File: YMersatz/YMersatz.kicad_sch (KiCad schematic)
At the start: 9 parts, among them J1 Conn_01x20, J2 Conn_01x20, U1 74LS574, U2 74LS08, Y1 SG-615

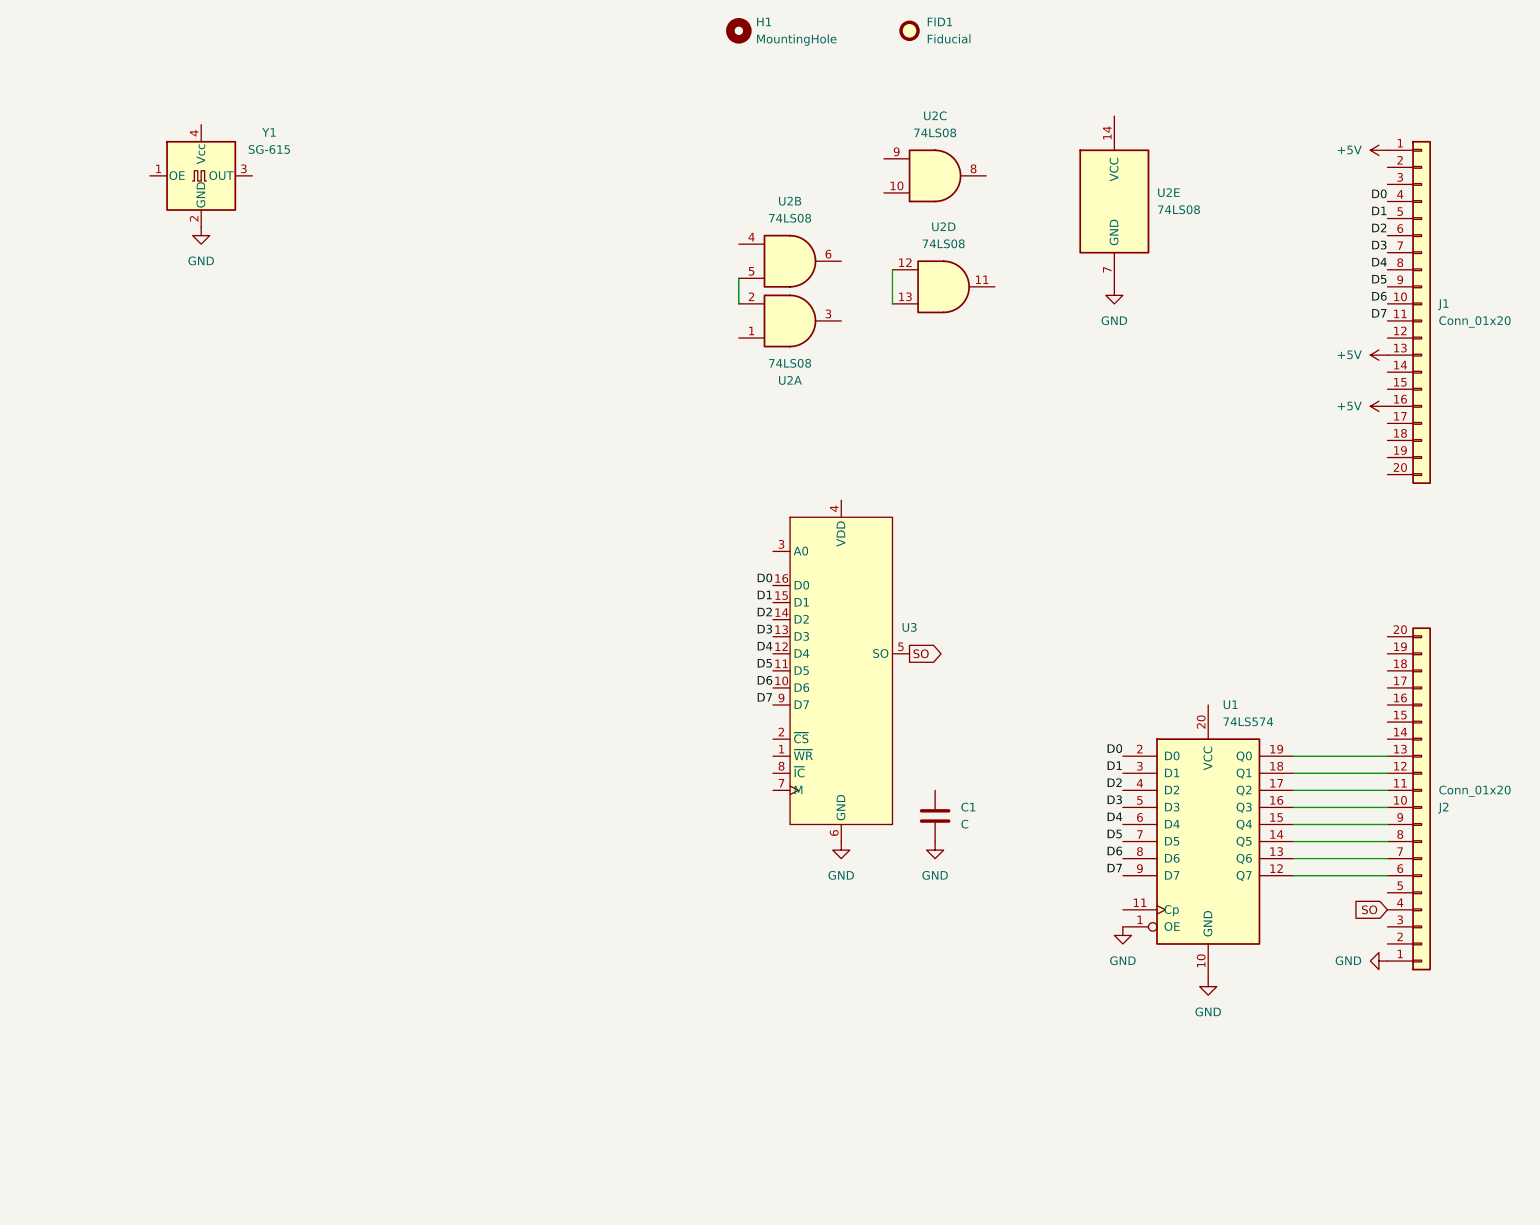
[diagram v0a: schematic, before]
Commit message: ym pins
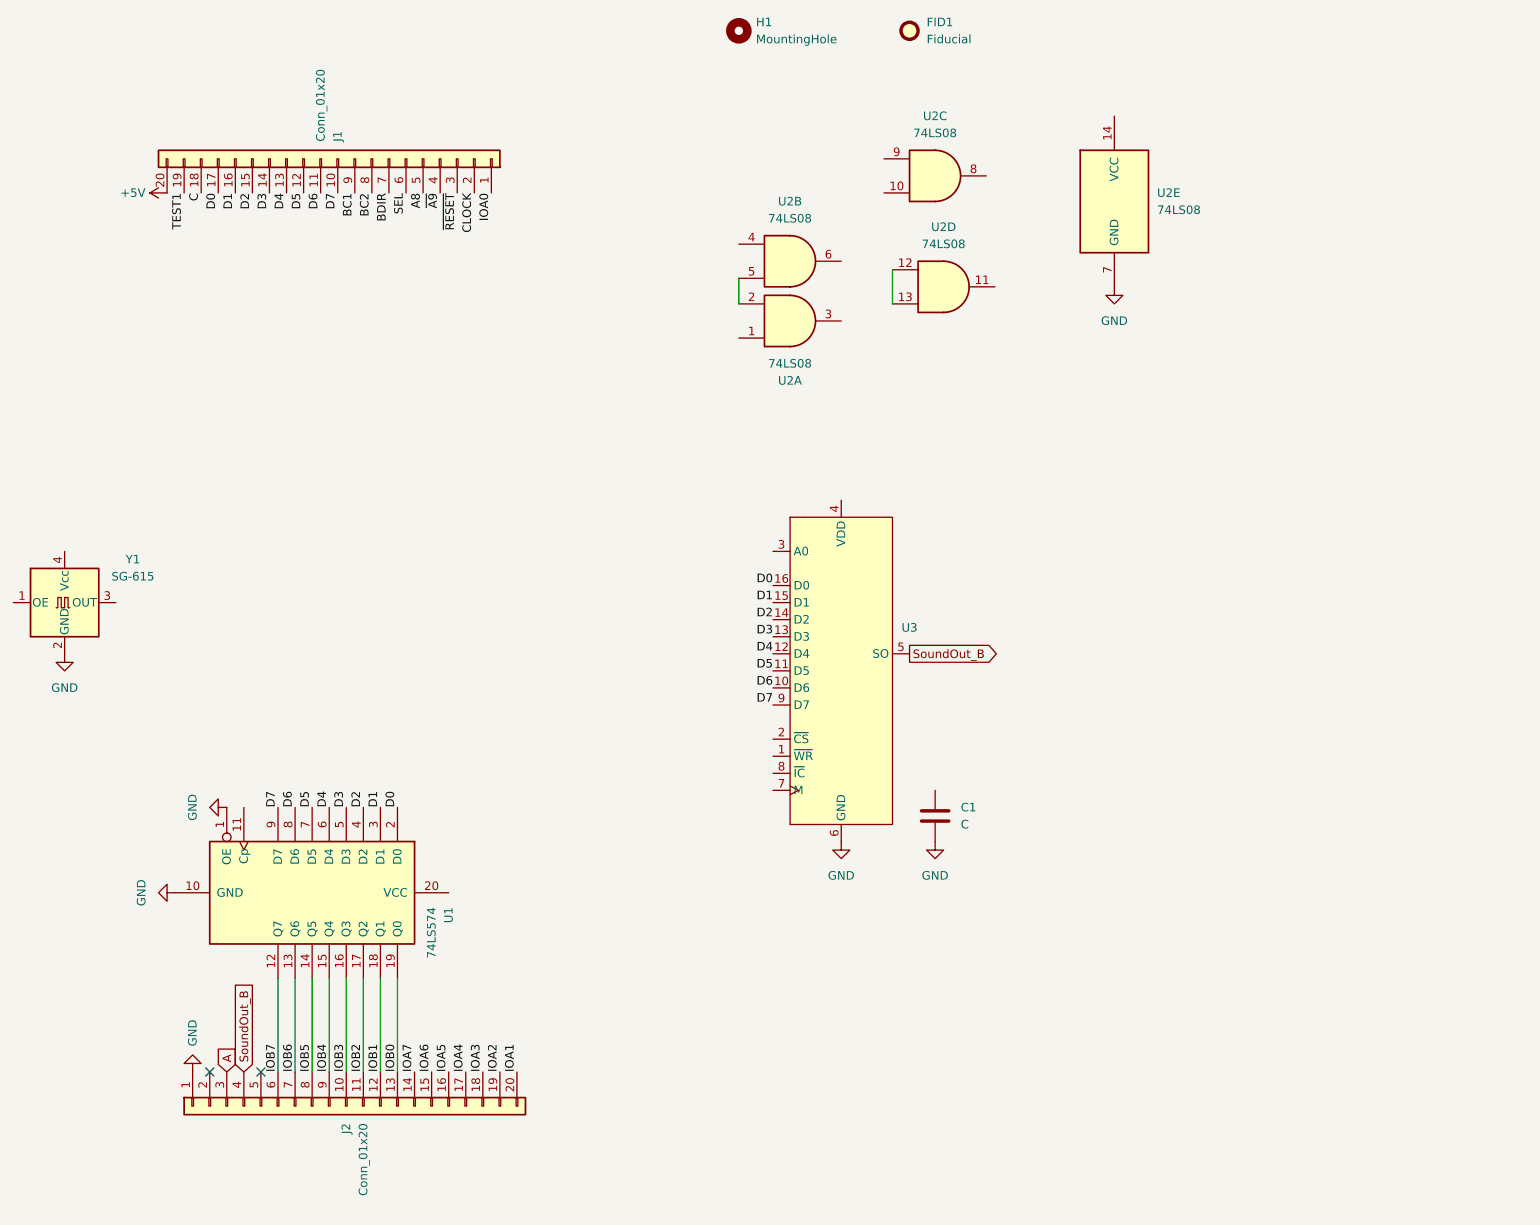
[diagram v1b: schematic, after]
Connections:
- net +5V: now also J1.20 (Pin_20); no longer J1.1 (Pin_1), J1.13 (Pin_13), J1.16 (Pin_16)
- net D0: now also J1.17 (Pin_17); no longer J1.4 (Pin_4)
- net D1: now also J1.16 (Pin_16); no longer J1.5 (Pin_5)
- net D2: now also J1.15 (Pin_15); no longer J1.6 (Pin_6)
- net D3: now also J1.14 (Pin_14); no longer J1.7 (Pin_7)
- net D4: now also J1.13 (Pin_13); no longer J1.8 (Pin_8)
- net D5: now also J1.12 (Pin_12); no longer J1.9 (Pin_9)
- net D6: now also J1.11 (Pin_11); no longer J1.10 (Pin_10)
- net D7: now also J1.10 (Pin_10); no longer J1.11 (Pin_11)
- net IOB7: now reaches J2.6 (Pin_6), U1.12 (Q7)
- net IOB6: now reaches J2.7 (Pin_7), U1.13 (Q6)
- net IOB5: now reaches J2.8 (Pin_8), U1.14 (Q5)
- net IOB4: now reaches J2.9 (Pin_9), U1.15 (Q4)
- net IOB3: now reaches J2.10 (Pin_10), U1.16 (Q3)
- net IOB2: now reaches J2.11 (Pin_11), U1.17 (Q2)
- net IOB1: now reaches J2.12 (Pin_12), U1.18 (Q1)
- net IOB0: now reaches J2.13 (Pin_13), U1.19 (Q0)
- net IOA7: now reaches J2.14 (Pin_14)
- net IOA6: now reaches J2.15 (Pin_15)
- net IOA5: now reaches J2.16 (Pin_16)
- net IOA4: now reaches J2.17 (Pin_17)
- net IOA3: now reaches J2.18 (Pin_18)
- net IOA2: now reaches J2.19 (Pin_19)
- net IOA1: now reaches J2.20 (Pin_20)
- net A: now reaches J2.3 (Pin_3)
- net C: now reaches J1.18 (Pin_18)
- net TEST1: now reaches J1.19 (Pin_19)
- net CLOCK: now reaches J1.2 (Pin_2)
- net ~{RESET}: now reaches J1.3 (Pin_3)
- net SO renamed SoundOut_B
- new net A8: J1.5 (Pin_5)
- new net BC1: J1.9 (Pin_9)
- new net BC2: J1.8 (Pin_8)
- new net BDIR: J1.7 (Pin_7)
- new net IOA0: J1.1 (Pin_1)
- new net SEL: J1.6 (Pin_6)
- new net ~{A9}: J1.4 (Pin_4)
- no-connect marks 0 -> 2
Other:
- moved on the sheet: J1, J2, U1, Y1
